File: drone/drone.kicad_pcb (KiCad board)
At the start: 2 copper layers, 53.3 x 55.2 mm, 52 parts, among them J3 Conn_01x03_Pin, SW1 SW_Push, SW2 SW_Push, U1 ESP32-WROOM-32D, U2 MPU-6050, U3 MP2303ADN

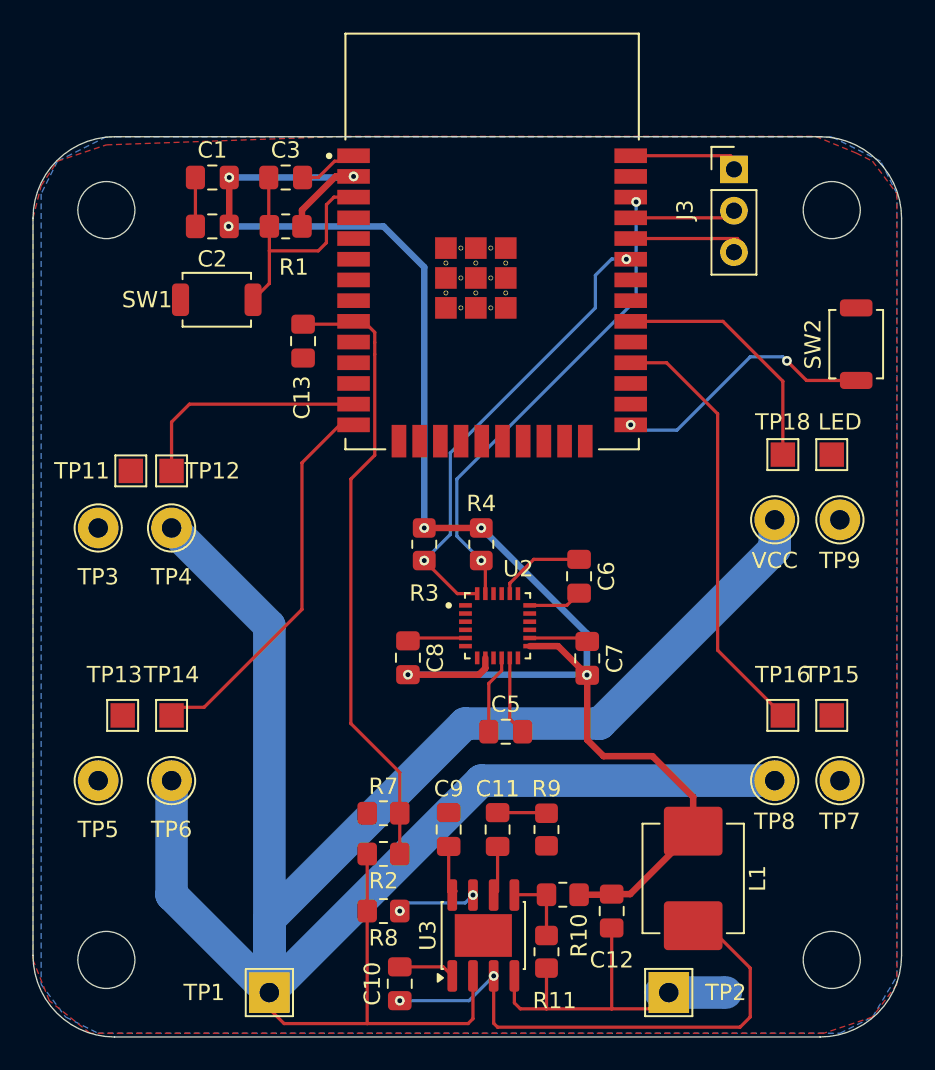
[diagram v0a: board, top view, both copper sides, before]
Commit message: hi
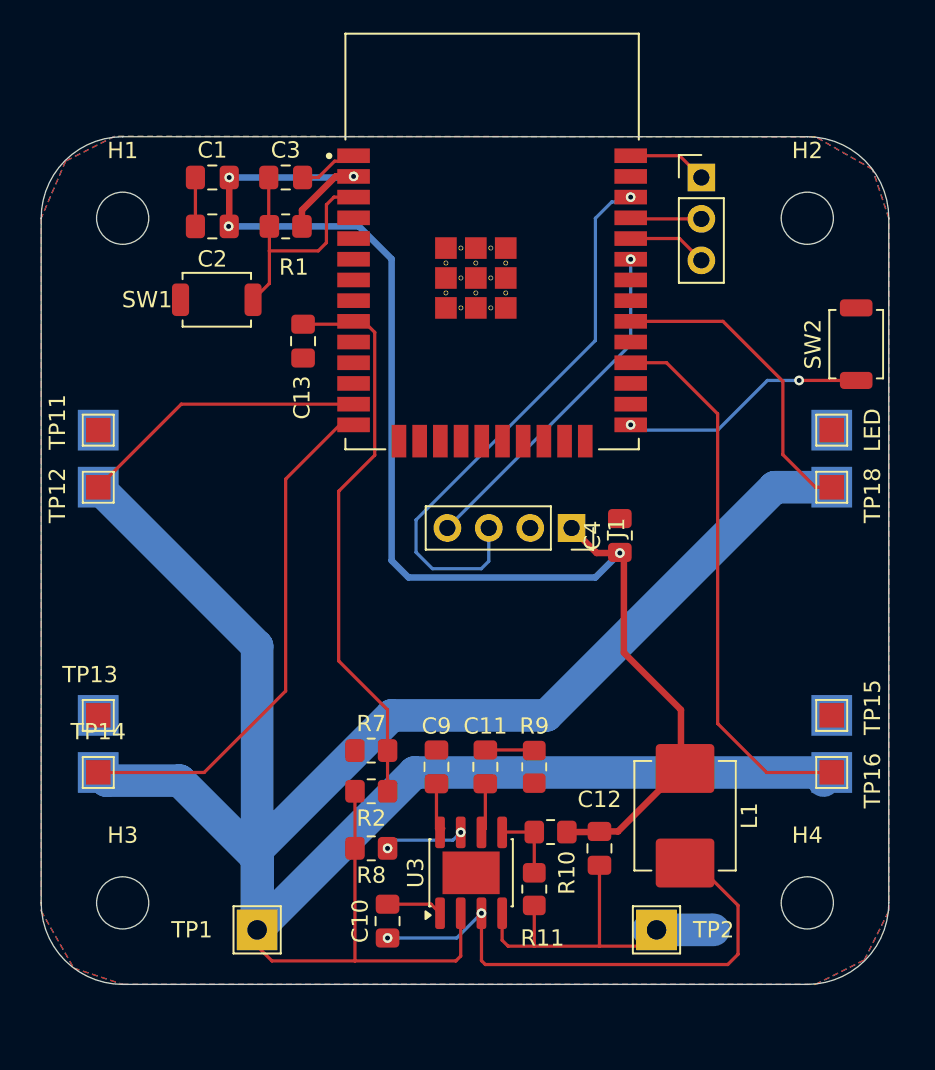
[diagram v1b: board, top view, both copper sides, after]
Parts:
- removed C5, C6: 220pF, Capacitor_SMD:C_0805_2012Metric_Pad1.18x1.45mm_HandSolder
- removed C7, C8: 0.1uF, Capacitor_SMD:C_0805_2012Metric_Pad1.18x1.45mm_HandSolder
- removed R3, R4: 4.7k, Resistor_SMD:R_0805_2012Metric_Pad1.20x1.40mm_HandSolder
- removed U2: MPU-6050, MPU-6050:QFN50P400X400X95-24N
- added C4: 10nF, Capacitor_SMD:C_0805_2012Metric_Pad1.18x1.45mm_HandSolder, F.Cu at (223.0, 94.5)
- added J1: Conn_01x04_Pin, Connector_PinSocket_2.54mm:PinSocket_1x04_P2.54mm_Vertical, F.Cu at (220.0, 94.0)
- H1, H2, H3, H4: footprint MountingHole:MountingHole_3.5mm -> MountingHole:MountingHole_3.2mm_M3
- TP10, TP3, TP4, TP5, TP6, TP7, TP8, TP9: footprint TestPoint:TestPoint_Pad_D2.5mm -> TestPoint:TestPoint_Pad_2.5x2.5mm; moved to B.Cu
- moved TP3 6.00 mm to (191.0, 88.0), turned to 180 degrees
- moved TP14 5.70 mm to (191.0, 109.0)
- moved TP9 5.52 mm to (236.0, 88.0), turned to 180 degrees
- moved TP4 5.15 mm to (191.0, 91.5), turned to 0 degrees
- moved TP12 4.61 mm to (191.0, 91.5)
- moved TP16 4.61 mm to (236.0, 109.0)
- moved TP6 4.53 mm to (191.0, 109.0), turned to 180 degrees
- moved TP10 4.03 mm to (236.0, 91.5), turned to 180 degrees
- moved TP7 4.03 mm to (236.0, 105.5), turned to 180 degrees
- moved TP5 4.00 mm to (191.0, 105.5), turned to 180 degrees
- moved C10 3.92 mm to (208.8, 118.1)
- moved C11 3.92 mm to (214.8, 108.7)
- moved C12 3.92 mm to (221.8, 113.7)
- moved C9 3.92 mm to (211.8, 108.7)
- moved NT1 3.92 mm to (226.8, 118.7)
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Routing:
- net GND: track 47.7 -> 30.7 mm
- net +3V3: track 103.9 -> 87.7 mm, vias 7 -> 4
- net ESC2: track 23.8 -> 32.1 mm
- net ESC VCC: track 156.1 -> 163.4 mm
- net SDA: track 28.3 -> 21.2 mm, vias 2 -> 1
- net ESC3: track 26.8 -> 33.9 mm
- net SCL: track 29.3 -> 34.9 mm, vias 2 -> 1
- net Net-(U2-CPOUT): track 5.49 -> 0.00 mm
- net Net-(U2-REGOUT): track 4.86 -> 0.00 mm
- net ESC4: track 15.4 -> 19.7 mm
- net Batt Read: track 39.1 -> 35.6 mm
- net ESC1: track 14.6 -> 17.8 mm
- net RX: track 7.70 -> 4.89 mm
- net TX: track 6.52 -> 4.36 mm
- net Net-(U1-IO0): track 16.9 -> 15.2 mm
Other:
- board size 53.3 x 55.2 mm -> 52 x 52 mm
